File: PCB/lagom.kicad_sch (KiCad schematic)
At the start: 165 parts

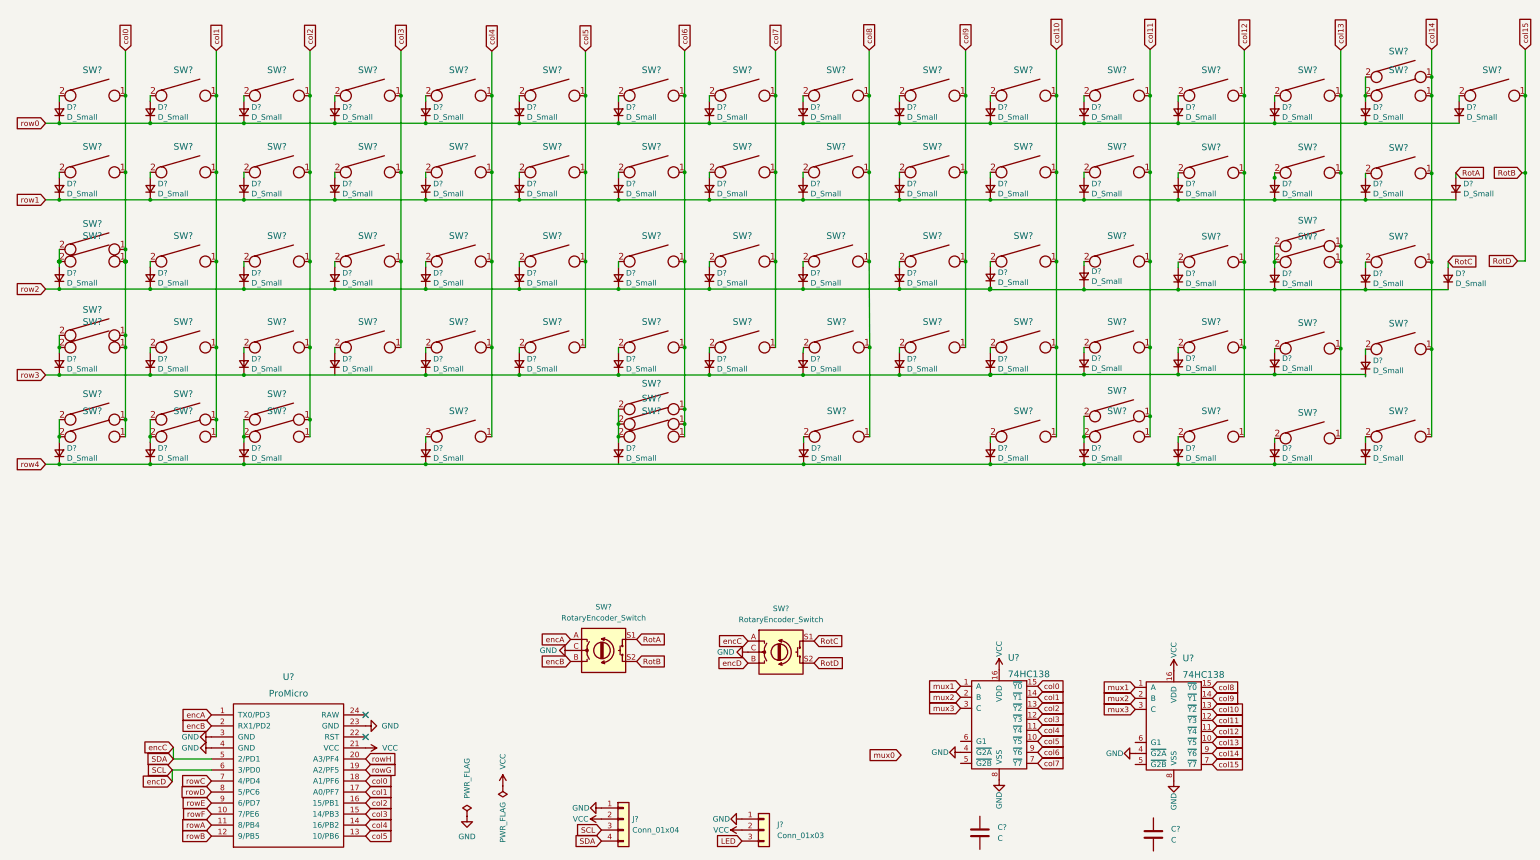
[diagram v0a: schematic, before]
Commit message: Schematic complete
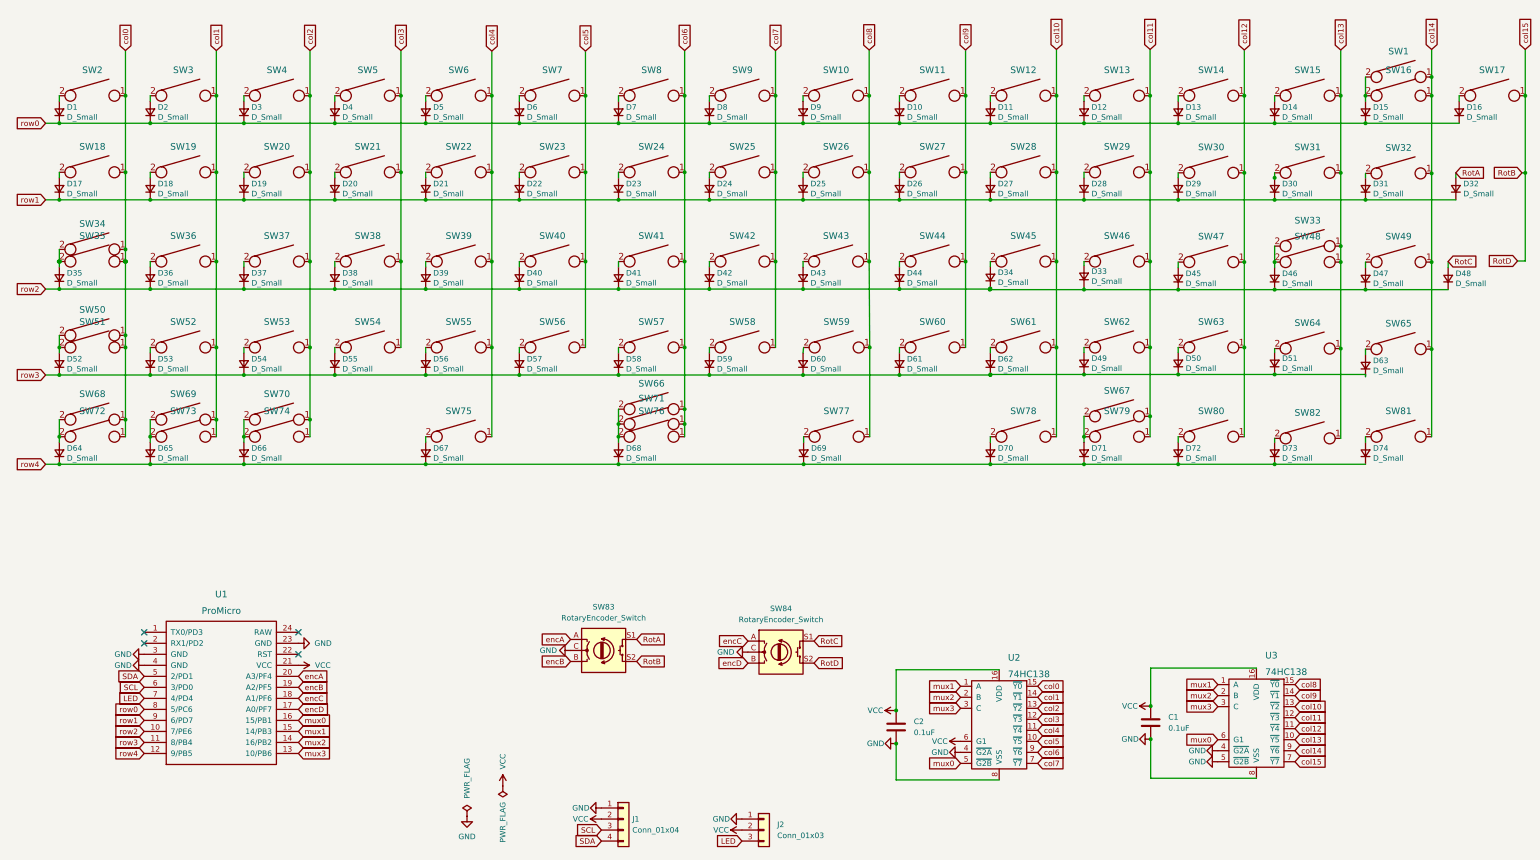
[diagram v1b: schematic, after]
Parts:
- C1, C2: renamed from C?; value C -> 0.1uF
- D1: renamed from D?; footprint Keebio-Parts:Diode -> Diode_THT:D_DO-35_SOD27_P7.62mm_Horizontal
- gave numbers to parts that had none: 162
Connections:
- net rowA is gone; now on net row3: U1.11 (8/PB4)
- net rowB is gone; now on net row4: U1.12 (9/PB5)
- net rowC is gone; now on net LED: U1.7 (4/PD4)
- net rowD is gone; now on net row0: U1.8 (5/PC6)
- net rowE is gone; now on net row1: U1.9 (6/PD7)
- net rowF is gone; now on net row2: U1.10 (7/PE6)
- net rowG is gone; now on net encB: U1.19 (A2/PF5)
- net rowH is gone; now on net encA: U1.20 (A3/PF4)
- net GND: now also C1.2, C2.2, U3.5 (~{G2B})
- net SCL: no longer SW84.B
- net SDA: no longer SW84.A
- net VCC: now also C1.1, C2.1, U2.6 (G1)
- net col0: no longer U1.18 (A1/PF6)
- net col1: no longer U1.17 (A0/PF7)
- net col2: no longer U1.16 (15/PB1)
- net col3: no longer U1.15 (14/PB3)
- net col4: no longer U1.14 (16/PB2)
- net col5: no longer U1.13 (10/PB6)
- net encA: no longer U1.1 (TX0/PD3)
- net encB: no longer U1.2 (RX1/PD2)
- net mux0: now also U1.16 (15/PB1), U2.5 (~{G2B}), U3.6 (G1)
- net mux1: now also U1.15 (14/PB3)
- net mux2: now also U1.14 (16/PB2)
- net mux3: now also U1.13 (10/PB6)
- net row3: now also D55.1 (K)
- net row4: now also D68.1 (K)
- new net encC: SW84.A, U1.18 (A1/PF6)
- new net encD: SW84.B, U1.17 (A0/PF7)
- no-connect marks 2 -> 4
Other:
- moved on the sheet: C1, C2, U1, U3

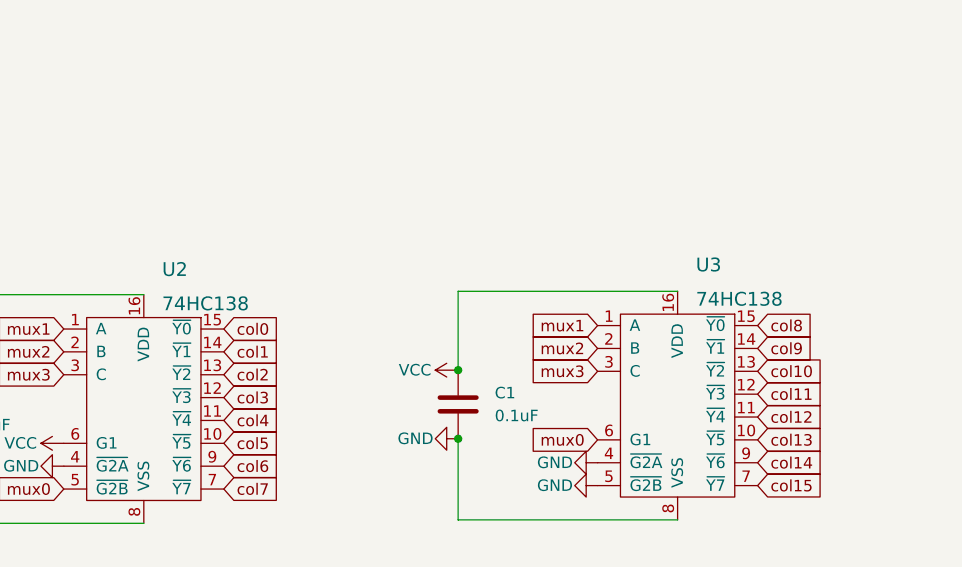
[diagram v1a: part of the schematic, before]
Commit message: PCB layout done
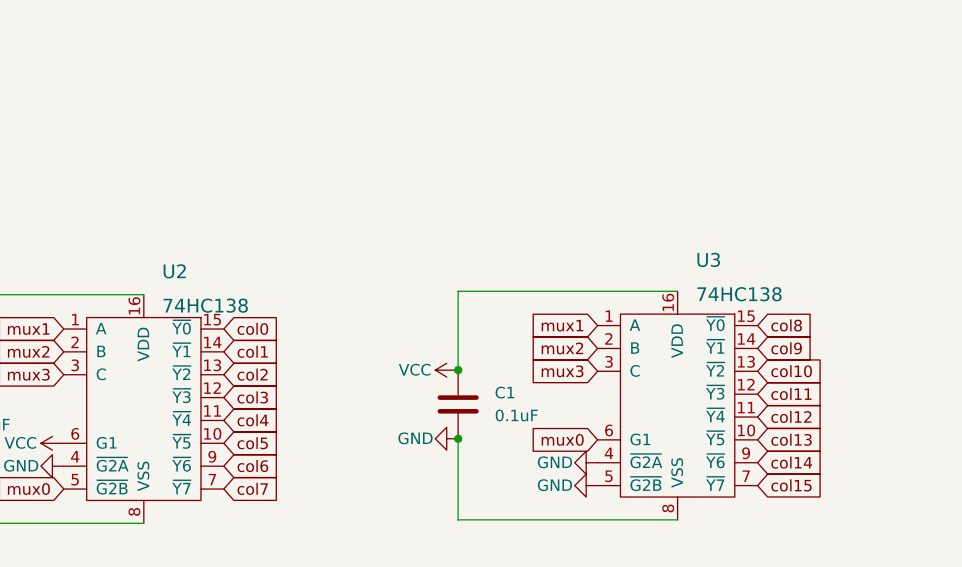
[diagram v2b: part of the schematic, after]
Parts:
- C1, C2: footprint (none) -> Capacitor_THT:C_Disc_D4.7mm_W2.5mm_P5.00mm
- J2: footprint (none) -> Connector_PinSocket_2.54mm:PinSocket_1x03_P2.54mm_Vertical
- SW13, SW17, SW29: footprint Button_Switch_Keyboard:SW_Cherry_MX_1.50u_PCB -> Button_Switch_Keyboard:SW_Cherry_MX_1.00u_PCB
- U2, U3: footprint (none) -> Package_DIP:DIP-16_W7.62mm_Socket
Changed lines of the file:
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@@
       (effects (font (size 1.27 1.27)) (justify left))
     )
-    (property "Footprint" "" (id 2) (at 246.8372 199.898 0)
+    (property "Footprint" "Capacitor_THT:C_Disc_D4.7mm_W2.5mm_P5.00mm" (id 2) (at 246.8372 199.898 0)
       (effects (font (size 1.27 1.27)) hide)
     )
@@
   (symbol (lib_id "w_logic:74HC138") (at 269.621 195.58 0) (unit 1)
     (in_bom yes) (on_board yes) (fields_autoplaced)
-    (property "Reference" "U2" (id 0) (at 271.6404 180.086 0)
+    (property "Reference" "U2" (id 0) (at 271.6404 180.34 0)
       (effects (font (size 1.524 1.524)) (justify left))
     )
-    (property "Value" "74HC138" (id 1) (at 271.6404 183.896 0)
+    (property "Value" "74HC138" (id 1) (at 271.6404 184.15 0)
       (effects (font (size 1.524 1.524)) (justify left))
     )
-    (property "Footprint" "" (id 2) (at 269.621 195.58 0)
-      (effects (font (size 1.524 1.524)))
+    (property "Footprint" "Package_DIP:DIP-16_W7.62mm_Socket" (id 2) (at 269.621 195.58 0)
+      (effects (font (size 1.524 1.524)) hide)
     )
     (property "Datasheet" "/mnt/dati/documenti/Elettronica/DATA_SHEET/Elettronici/Integrati/Digitali/Registri/NXP_74HC138_74HCT138.pdf" (id 3) (at 271.6404 183.896 0)
@@
       (effects (font (size 1.524 1.524)) hide)
     )
-    (property "Footprint" "Button_Switch_Keyboard:SW_Cherry_MX_1.50u_PCB" (id 2) (at 383.286 50.546 0)
+    (property "Footprint" "Button_Switch_Keyboard:SW_Cherry_MX_1.00u_PCB" (id 2) (at 383.286 50.546 0)
       (effects (font (size 1.524 1.524)) hide)
     )
@@
       (effects (font (size 1.524 1.524)) hide)
     )
-    (property "Footprint" "Button_Switch_Keyboard:SW_Cherry_MX_1.50u_PCB" (id 2) (at 296.799 50.546 0)
+    (property "Footprint" "Button_Switch_Keyboard:SW_Cherry_MX_1.00u_PCB" (id 2) (at 296.799 50.546 0)
       (effects (font (size 1.524 1.524)) hide)
     )
@@
       (effects (font (size 1.27 1.27)) (justify left))
     )
-    (property "Footprint" "" (id 2) (at 215.392 219.837 0)
+    (property "Footprint" "Connector_PinSocket_2.54mm:PinSocket_1x03_P2.54mm_Vertical" (id 2) (at 215.392 219.837 0)
       (effects (font (size 1.27 1.27)) hide)
     )
@@
       (effects (font (size 1.27 1.27)) (justify left))
     )
-    (property "Footprint" "" (id 2) (at 305.5112 198.882 0)
+    (property "Footprint" "Capacitor_THT:C_Disc_D4.7mm_W2.5mm_P5.00mm" (id 2) (at 305.5112 198.882 0)
       (effects (font (size 1.27 1.27)) hide)
     )
@@
   (symbol (lib_id "w_logic:74HC138") (at 328.93 195.199 0) (unit 1)
     (in_bom yes) (on_board yes) (fields_autoplaced)
-    (property "Reference" "U3" (id 0) (at 330.9494 179.578 0)
+    (property "Reference" "U3" (id 0) (at 330.9494 179.07 0)
       (effects (font (size 1.524 1.524)) (justify left))
     )
-    (property "Value" "74HC138" (id 1) (at 330.9494 183.388 0)
+    (property "Value" "74HC138" (id 1) (at 330.9494 182.88 0)
       (effects (font (size 1.524 1.524)) (justify left))
     )
-    (property "Footprint" "" (id 2) (at 328.93 195.199 0)
-      (effects (font (size 1.524 1.524)))
+    (property "Footprint" "Package_DIP:DIP-16_W7.62mm_Socket" (id 2) (at 328.93 195.199 0)
+      (effects (font (size 1.524 1.524)) hide)
     )
     (property "Datasheet" "/mnt/dati/documenti/Elettronica/DATA_SHEET/Elettronici/Integrati/Digitali/Registri/NXP_74HC138_74HCT138.pdf" (id 3) (at 330.9494 183.515 0)
@@
       (effects (font (size 1.524 1.524)) hide)
     )
-    (property "Footprint" "Button_Switch_Keyboard:SW_Cherry_MX_1.50u_PCB" (id 2) (at 296.799 68.199 0)
+    (property "Footprint" "Button_Switch_Keyboard:SW_Cherry_MX_1.00u_PCB" (id 2) (at 296.799 68.199 0)
       (effects (font (size 1.524 1.524)) hide)
     )
@@
     )
     (path "/bc00cb6d-ff28-45b9-b930-be73b03fd96d"
-      (reference "C1") (unit 1) (value "0.1uF") (footprint "")
+      (reference "C1") (unit 1) (value "0.1uF") (footprint "Capacitor_THT:C_Disc_D4.7mm_W2.5mm_P5.00mm")
     )
     (path "/0fd8c6ab-3384-49aa-8e48-3f4df84bc20e"
-      (reference "C2") (unit 1) (value "0.1uF") (footprint "")
+      (reference "C2") (unit 1) (value "0.1uF") (footprint "Capacitor_THT:C_Disc_D4.7mm_W2.5mm_P5.00mm")
     )
     (path "/afa695ae-8ccf-42d3-9dcb-5e731da4e36c"
@@
     )
     (path "/afffe1fe-d14c-481c-bd58-ae7a8ca3d519"
-      (reference "J2") (unit 1) (value "Conn_01x03") (footprint "")
+      (reference "J2") (unit 1) (value "Conn_01x03") (footprint "Connector_PinSocket_2.54mm:PinSocket_1x03_P2.54mm_Vertical")
     )
     (path "/a5c5762f-a0e0-401e-8bc4-621198606bcb"
@@
     )
     (path "/9c21fdb3-4254-429a-8fa6-c29cf995b177"
-      (reference "SW13") (unit 1) (value "KEYSW") (footprint "Button_Switch_Keyboard:SW_Cherry_MX_1.50u_PCB")
+      (reference "SW13") (unit 1) (value "KEYSW") (footprint "Button_Switch_Keyboard:SW_Cherry_MX_1.00u_PCB")
     )
     (path "/fec9eaae-d6bc-4df4-9d8e-a08e2c64f06c"
@@
     )
     (path "/9808b20e-3499-4769-b8e9-46d57a37bd43"
-      (reference "SW17") (unit 1) (value "KEYSW") (footprint "Button_Switch_Keyboard:SW_Cherry_MX_1.50u_PCB")
+      (reference "SW17") (unit 1) (value "KEYSW") (footprint "Button_Switch_Keyboard:SW_Cherry_MX_1.00u_PCB")
     )
     (path "/05d4fb02-3c60-405c-9080-fb8446959d7e"
@@
     )
     (path "/e9fcf385-9380-4c87-8aca-dfe9bbcc7460"
-      (reference "SW29") (unit 1) (value "KEYSW") (footprint "Button_Switch_Keyboard:SW_Cherry_MX_1.50u_PCB")
+      (reference "SW29") (unit 1) (value "KEYSW") (footprint "Button_Switch_Keyboard:SW_Cherry_MX_1.00u_PCB")
     )
     (path "/71d08102-98f4-4a2d-8663-96fe9600f004"
@@
     )
     (path "/6894fe82-0ee5-4f27-a435-6dbd0d79b968"
-      (reference "U2") (unit 1) (value "74HC138") (footprint "")
+      (reference "U2") (unit 1) (value "74HC138") (footprint "Package_DIP:DIP-16_W7.62mm_Socket")
     )
     (path "/c92f95b2-2642-46df-8ce4-131bc603da4f"
-      (reference "U3") (unit 1) (value "74HC138") (footprint "")
+      (reference "U3") (unit 1) (value "74HC138") (footprint "Package_DIP:DIP-16_W7.62mm_Socket")
     )
   )
